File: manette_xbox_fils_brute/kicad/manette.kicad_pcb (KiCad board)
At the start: 2 copper layers, 106 x 74 mm, 31 parts, among them J1 THB001P, J2 THB001P, J3 Conn_01x20, X1 SW_Push, Y1 SW_Push

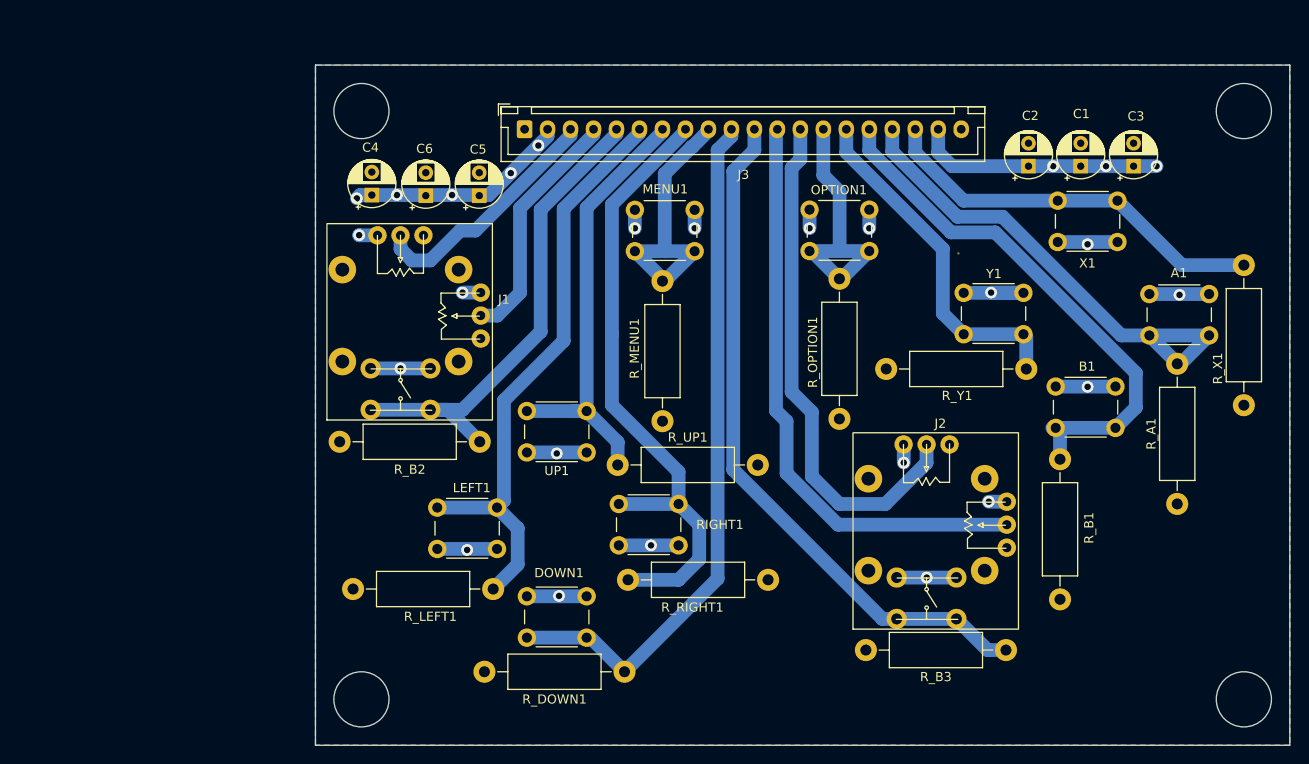
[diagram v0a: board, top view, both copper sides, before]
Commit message: redimensionnement de la carte
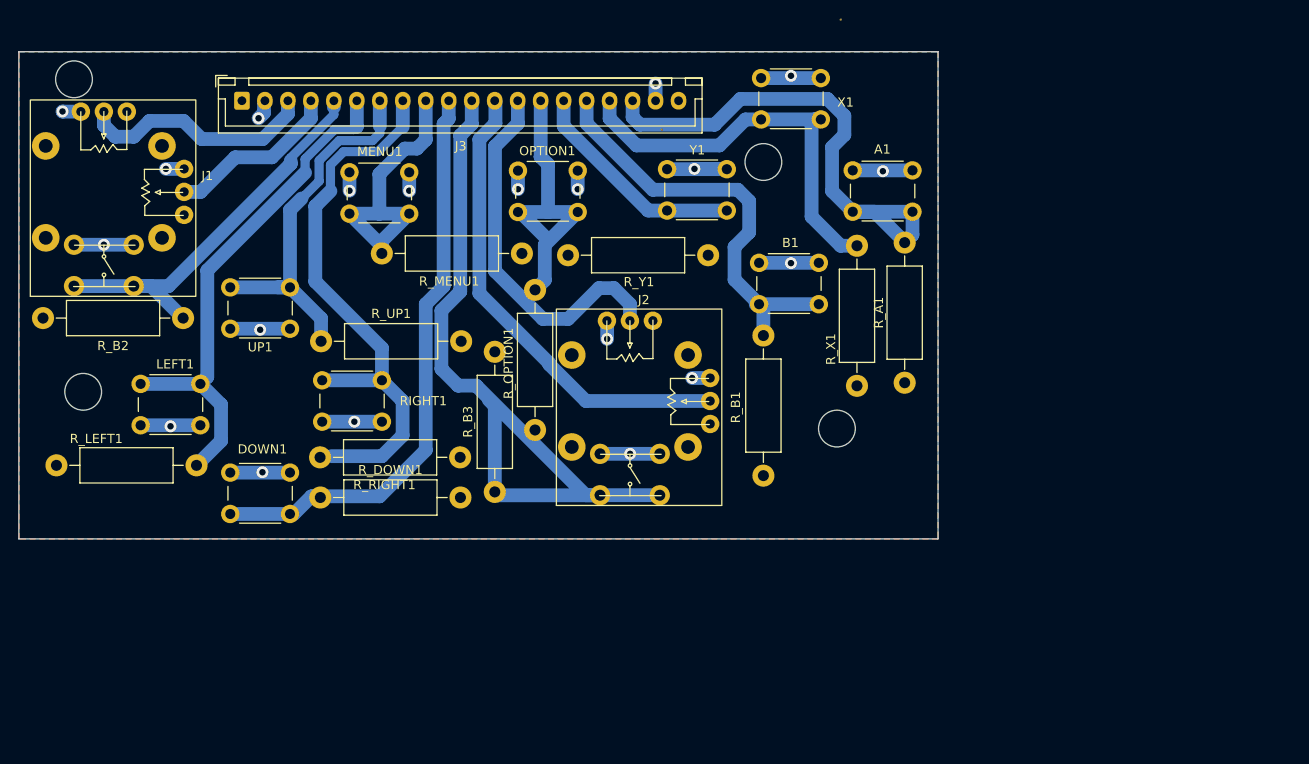
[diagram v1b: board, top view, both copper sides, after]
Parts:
- removed C1, C4: 100p, Capacitor_THT:CP_Radial_D5.0mm_P2.50mm
- removed C2, C5: 100n, Capacitor_THT:CP_Radial_D5.0mm_P2.50mm
- removed C3, C6: 10m, Capacitor_THT:CP_Radial_D5.0mm_P2.50mm
- moved R_B3 51.8 mm to (150.5, 103.2), turned to -90 degrees
- moved X1 42.7 mm to (179.5, 73.4), turned to 0 degrees
- moved R_X1 42.1 mm to (189.9, 106.9)
- moved R_Y1 36.8 mm to (158.5, 92.7)
- moved R_RIGHT1 36.1 mm to (131.5, 114.7)
- moved B1 35.0 mm to (185.8, 98.0)
- moved RIGHT1 35.0 mm to (138.2, 110.8)
- moved R_B1 35.0 mm to (179.7, 116.7)
- moved R_LEFT1 35.0 mm to (102.8, 115.5)
- moved R_UP1 35.0 mm to (146.8, 102.0)
- moved UP1 35.0 mm to (128.2, 100.7)
- moved Y1 35.0 mm to (175.8, 87.8)
- moved A1 35.0 mm to (189.4, 83.5)
- moved DOWN1 35.0 mm to (128.2, 120.8)
- moved J1 35.0 mm to (108.0, 85.8)
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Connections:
- J3 pad 17: A -> X
- J3 pad 18: X -> A
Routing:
- net JOY_B_X: track 56.7 -> 0.00 mm
- net 5V: track 135.8 -> 88.6 mm, vias 26 -> 20
- net OPTION: track 29.5 -> 73.9 mm
- net Y: track 38.4 -> 24.3 mm
- net DOWN: track 76.0 -> 63.2 mm
- net JOY_B_Y: track 64.2 -> 51.7 mm
- net B: track 58.7 -> 47.1 mm
- net JOY_A_A: track 54.3 -> 44.7 mm
- net LEFT: track 65.0 -> 56.5 mm
- net UP: track 49.2 -> 41.6 mm
- net RIGHT: track 69.2 -> 61.7 mm
- net JOY_A_Y: track 26.4 -> 19.0 mm
- net JOY_B_A: track 75.8 -> 81.9 mm
- net A: track 54.3 -> 56.3 mm
- net X: track 43.3 -> 45.0 mm
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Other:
- board size 106 x 74 mm -> 100 x 53 mm
